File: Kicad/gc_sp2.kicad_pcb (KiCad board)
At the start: 2 copper layers, 36.5 x 19.5 mm, 3 parts, among them J1 Micro_SD_Card, P1 SerialPort

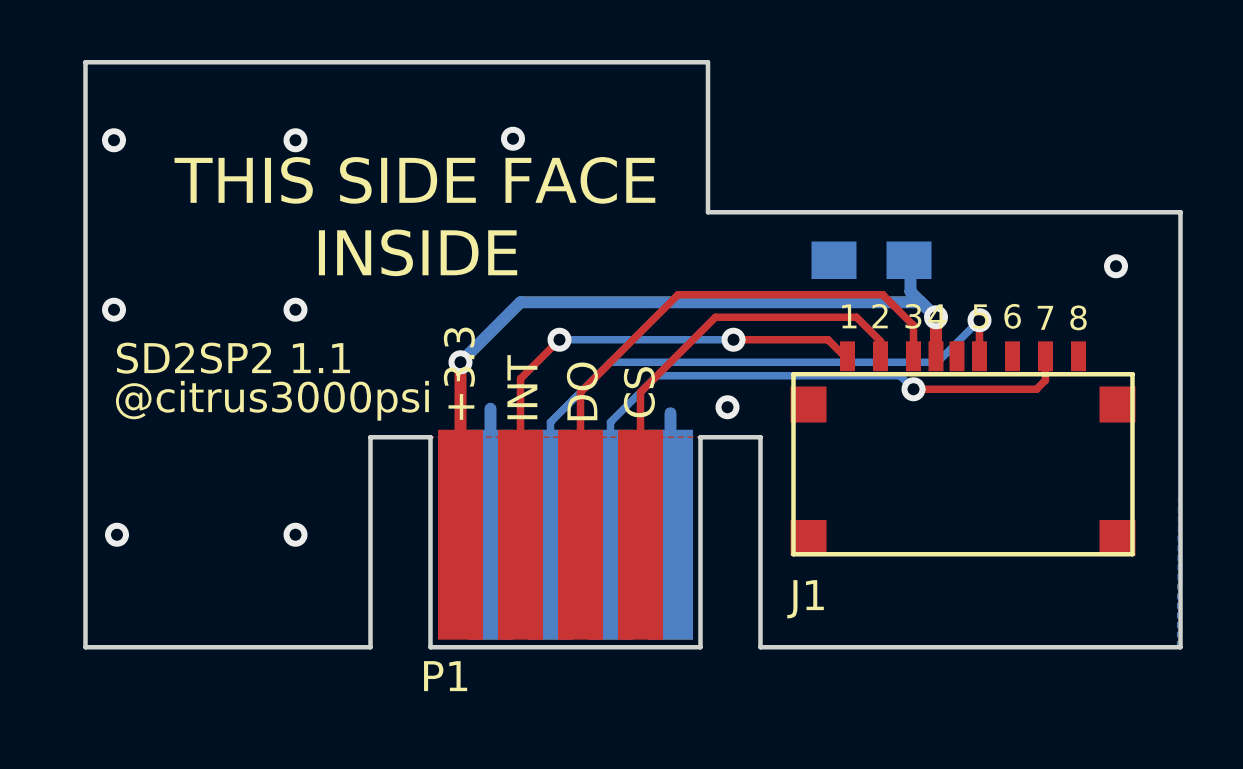
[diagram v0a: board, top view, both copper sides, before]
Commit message: Updated Design
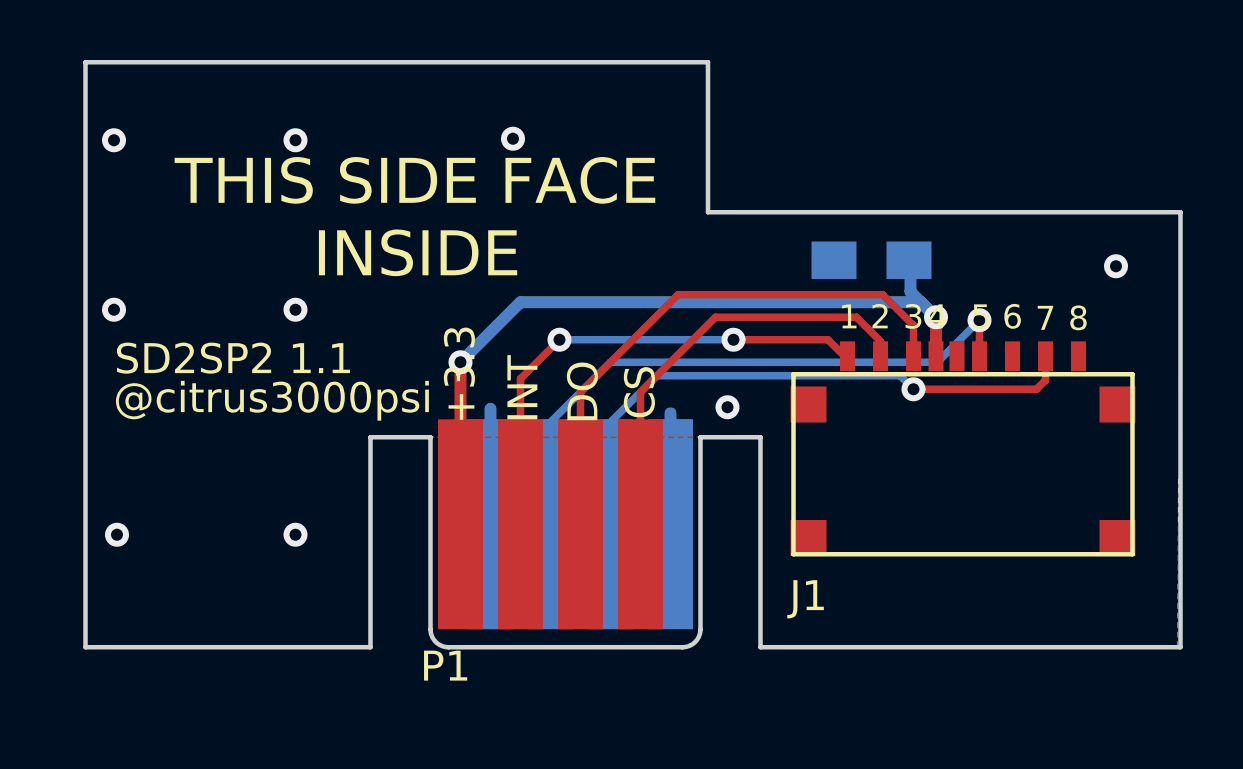
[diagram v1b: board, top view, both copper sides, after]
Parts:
- moved P1 0.35 mm to (75.5, 115.9)
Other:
- outline, holes or cut-outs redrawn
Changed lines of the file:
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@@
-(kicad_pcb (version 20171130) (host pcbnew "(5.0.0)")
+(kicad_pcb (version 20171130) (host pcbnew "(5.1.0)-1")
   (general
     (thickness 1.2)
-    (drawings 34)
+    (drawings 36)
     (tracks 53)
     (zones 0)
@@
     (36 B.SilkS user)
     (37 F.SilkS user)
-    (38 B.Mask user)
+    (38 B.Mask user hide)
     (39 F.Mask user)
     (40 Dwgs.User user)
@@
     (zone_45_only no)
     (trace_min 0.2)
-    (segment_width 0.2)
-    (edge_width 0.15)
     (via_size 0.8)
     (via_drill 0.4)
@@
     (uvia_min_size 0.2)
     (uvia_min_drill 0.1)
+    (edge_width 0.15)
+    (segment_width 0.2)
     (pcb_text_width 0.3)
     (pcb_text_size 1.5 1.5)
@@
   )
   (module gc_sp2:SP2_FootPrint (layer F.Cu)
-    (at 75.5 116.25)
+    (at 75.5 115.9)
     (fp_text reference P1 (at -0.5 4.75) (layer F.SilkS)
       (effects (font (size 1 1) (thickness 0.15)))
@@
     )
   )
+  (gr_arc (start 75.1 119.4) (end 74.5 119.4) (angle -90) (layer Edge.Cuts) (width 0.15))
+  (gr_arc (start 82.9 119.4) (end 82.9 120) (angle -90) (layer Edge.Cuts) (width 0.15))
   (gr_text DI (at 80.5 111.6 90) (layer B.SilkS)
     (effects (font (size 1 1) (thickness 0.15)) (justify mirror))
@@
     (effects (font (size 1.5 1.5) (thickness 0.3)))
   )
-  (gr_line (start 74.5 120) (end 83.5 120) (layer Edge.Cuts) (width 0.15))
-  (gr_line (start 74.5 113) (end 74.5 120) (layer Edge.Cuts) (width 0.15))
+  (gr_line (start 75.1 120) (end 82.9 120) (layer Edge.Cuts) (width 0.15))
+  (gr_line (start 74.5 113) (end 74.5 119.4) (layer Edge.Cuts) (width 0.15))
   (gr_line (start 72.5 113) (end 74.5 113) (layer Edge.Cuts) (width 0.15))
-  (gr_line (start 83.5 113) (end 83.5 120) (layer Edge.Cuts) (width 0.15))
+  (gr_line (start 83.5 113) (end 83.5 119.4) (layer Edge.Cuts) (width 0.15))
   (gr_line (start 83.5 113) (end 85.5 113) (layer Edge.Cuts) (width 0.15))
   (gr_line (start 85.5 120) (end 85.5 113) (layer Edge.Cuts) (width 0.15))
@@
   (segment (start 92.8 109.1) (end 91.4 110.5) (width 0.25) (layer B.Cu) (net 4))
   (segment (start 91.4 110.5) (end 80.5 110.5) (width 0.25) (layer B.Cu) (net 4))
-  (segment (start 79.5 111.5) (end 82.75 108.25) (width 0.25) (layer F.Cu) (net 6))
-  (segment (start 79.5 116.25) (end 79.5 111.5) (width 0.25) (layer F.Cu) (net 6))
   (via (at 90.6 111.4) (size 0.8) (drill 0.4) (layers F.Cu B.Cu) (net 5))
   (segment (start 80.5 112.5) (end 80.5 116.25) (width 0.25) (layer B.Cu) (net 5))
@@
   (segment (start 95 111.1) (end 95 110.3) (width 0.25) (layer F.Cu) (net 5))
   (segment (start 94.7 111.4) (end 95 111.1) (width 0.25) (layer F.Cu) (net 5))
+  (segment (start 79.5 111.5) (end 82.75 108.25) (width 0.25) (layer F.Cu) (net 6))
+  (segment (start 79.5 116.25) (end 79.5 111.5) (width 0.25) (layer F.Cu) (net 6))
   (segment (start 90.6 110.3) (end 90.6 109.275) (width 0.25) (layer F.Cu) (net 6))
   (segment (start 89.575 108.25) (end 82.75 108.25) (width 0.25) (layer F.Cu) (net 6))
